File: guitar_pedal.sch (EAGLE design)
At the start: 89 parts, among them P1 RM-065, P2 RM-065, P3 RM-065, U1 LM324N, U2 LM324N, U3 LM386N-3, U4 LM386N-3, U5 LM386N-3

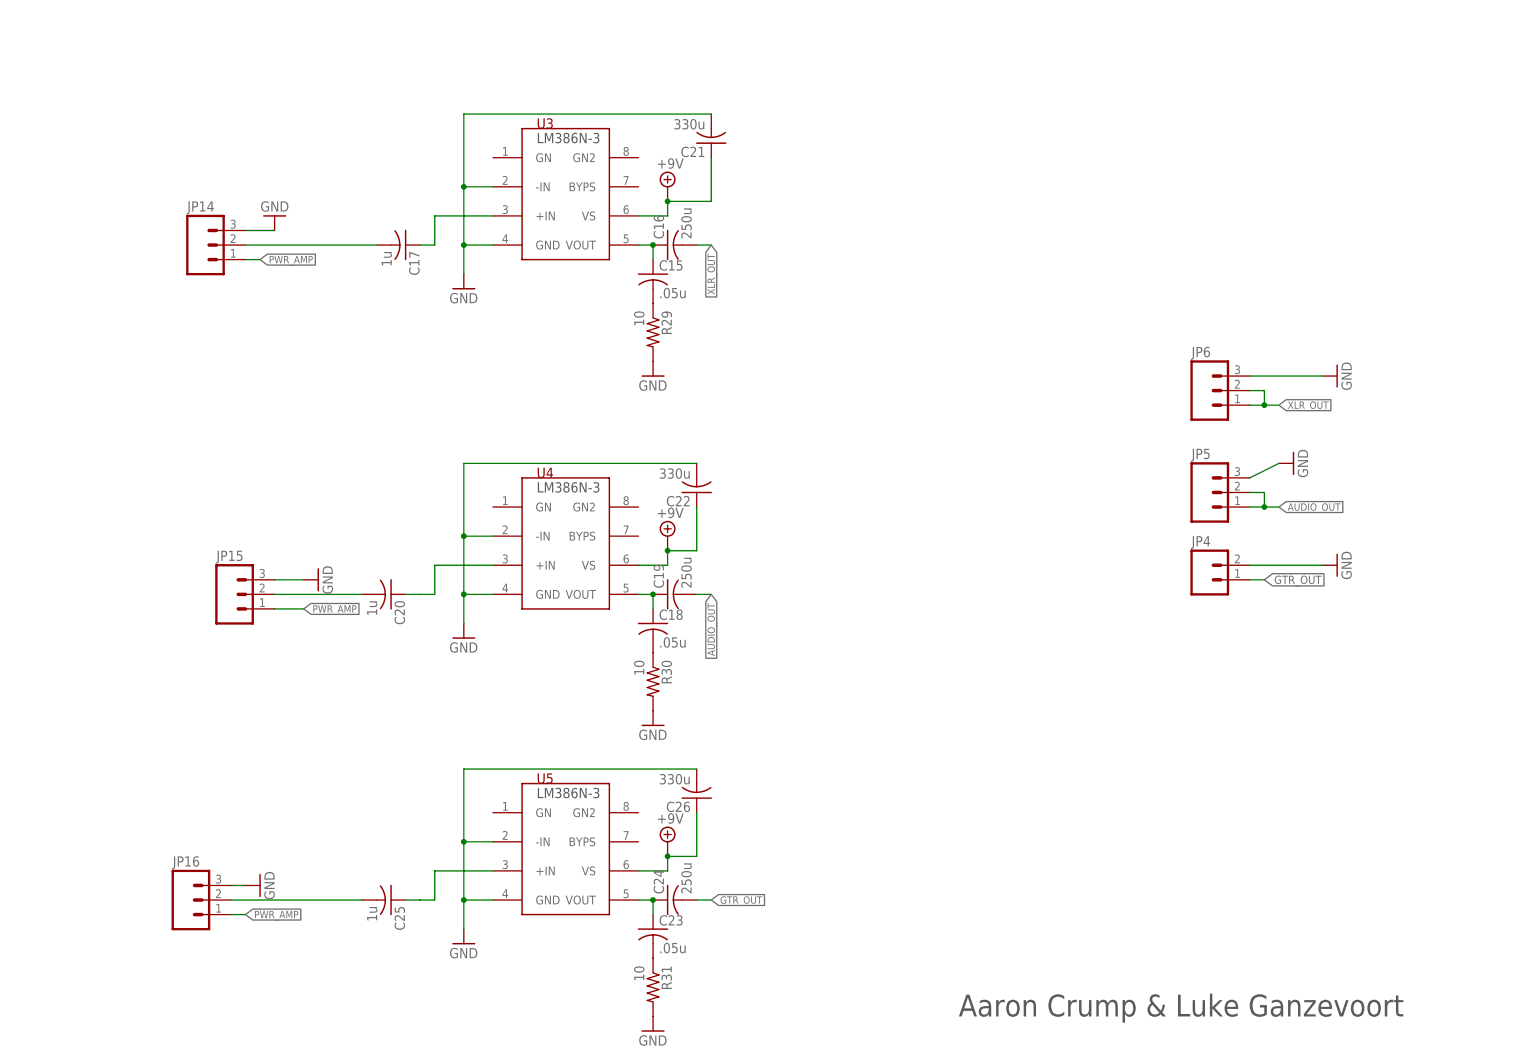
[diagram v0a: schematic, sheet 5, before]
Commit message: Finished organizing sheets
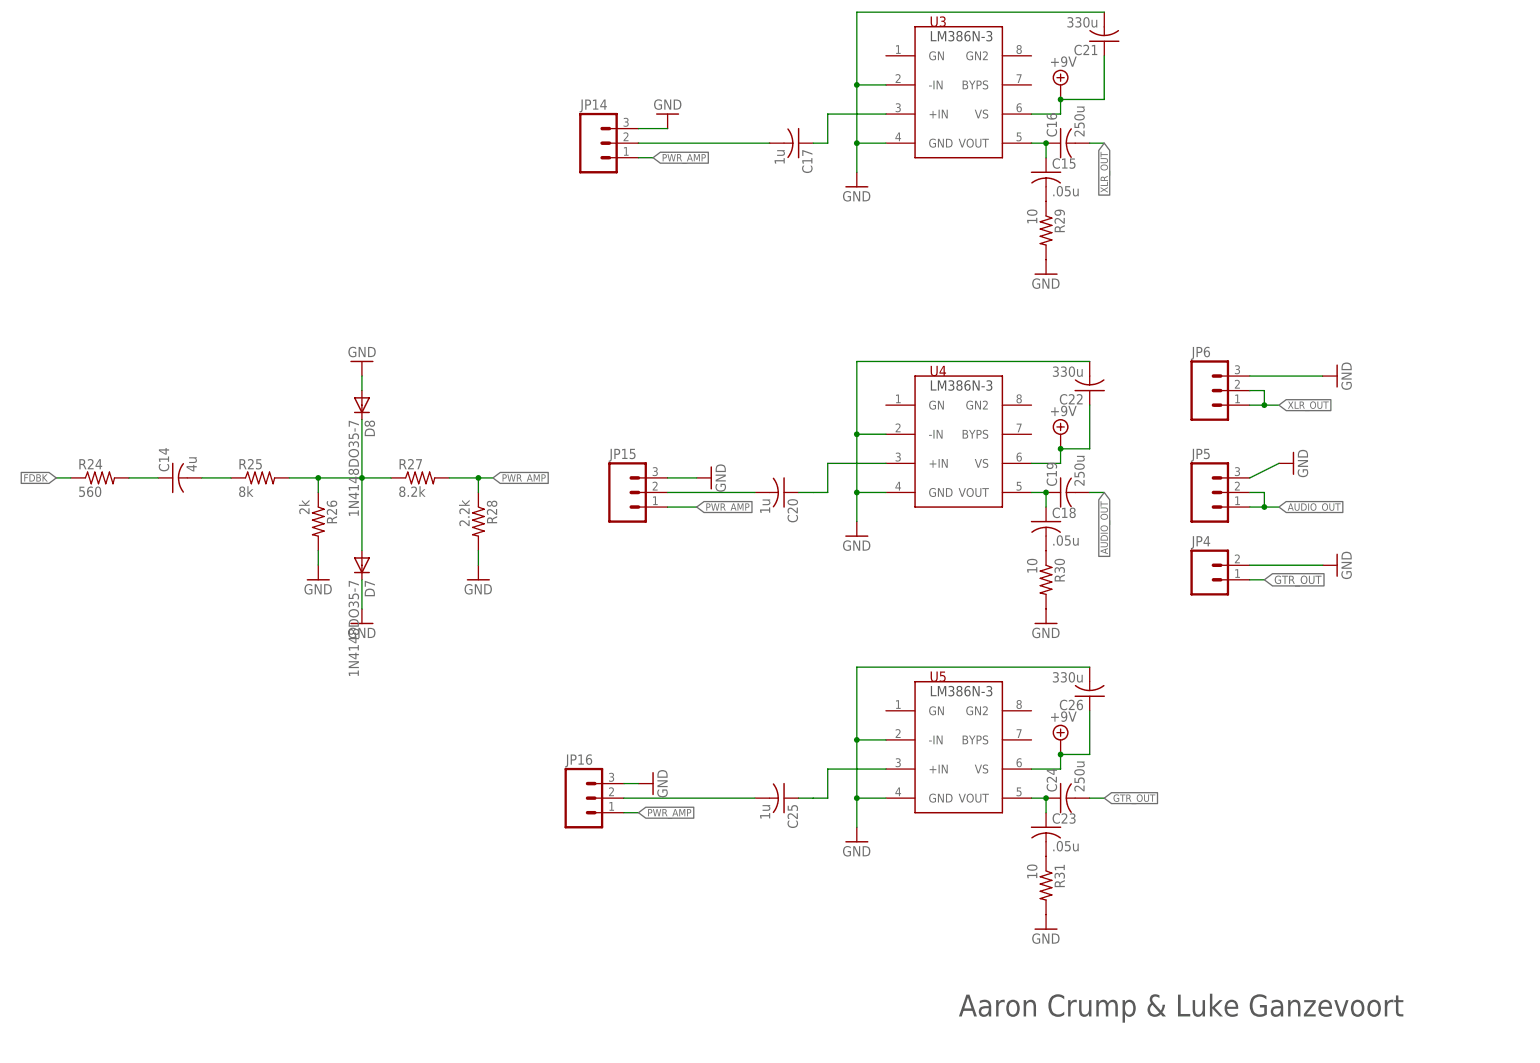
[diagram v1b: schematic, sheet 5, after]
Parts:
- C1, C2: value 100uF -> 100u
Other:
- moved on the sheet: C15, C16, C17, C18, C19, C20, C21, C22, C23, C24, C25, C26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
